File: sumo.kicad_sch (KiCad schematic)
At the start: 51 parts, among them Q1 BPW40, Q2 BPW40, SW1 SW_Push, SW2 SW_DIP_x01, T1 Screw_Terminal_01x04, T2 Screw_Terminal_01x04, T3 Screw_Terminal_01x04, T4 Screw_Terminal_01x04, T5 Screw_Terminal_01x04, U1 PIC16F628A-IP, U2 L7805, U3 L293D, U4 74HC04, U5 TSOP4038, U6 TSOP4038

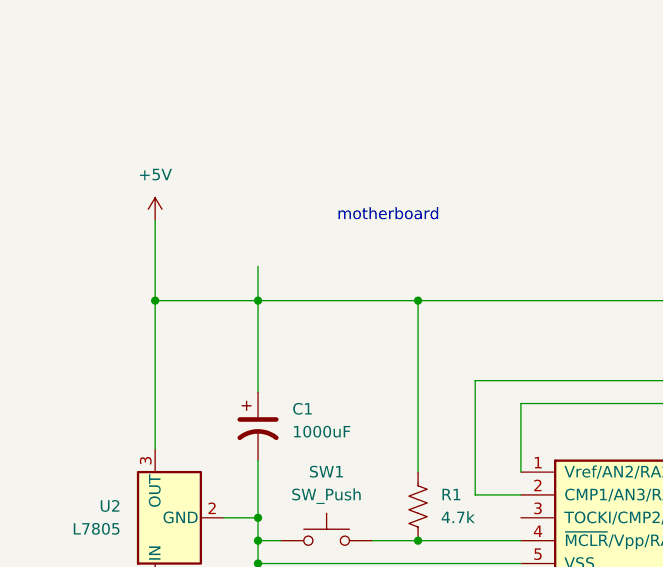
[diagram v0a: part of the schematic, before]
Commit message: motor driver
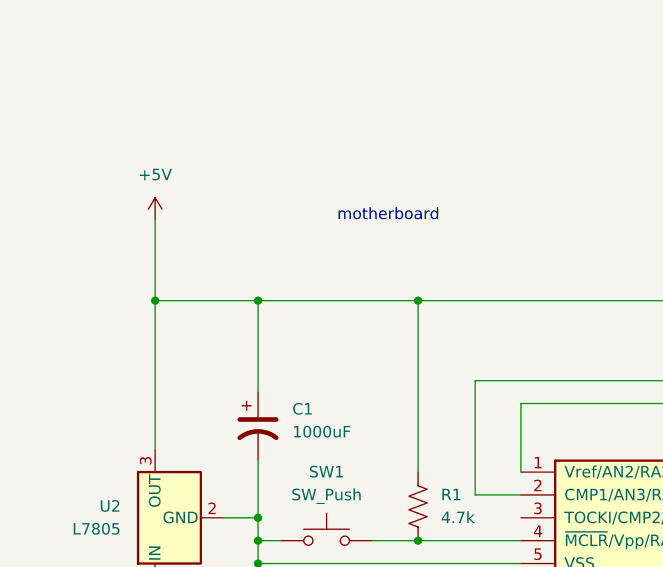
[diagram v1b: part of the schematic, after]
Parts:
- BT1, BT2, BT3: footprint (none) -> Battery:Battery_Pads
- C1: footprint Button_Switch_THT:SW_PUSH_1P1T_6x3.5mm_H5.0_APEM_MJTP1250 -> Capacitor_THT:C_Radial_D10.0mm_H12.5mm_P5.00mm
- SW2: footprint Button_Switch_SMD:SW_DIP_SPSTx01_Slide_9.78x4.72mm_W8.61mm_P2.54mm -> Button_Switch_THT:SW_DIP_SPSTx01_Slide_9.78x4.72mm_W7.62mm_P2.54mm
- T1, T2, T3, T4, T5: footprint TerminalBlock:TerminalBlock_bornier-4_P5.08mm -> TerminalBlock_MetzConnect:TerminalBlock_MetzConnect_Type086_RT03404HBLC_1x04_P3.81mm_Horizontal
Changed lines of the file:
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@@
 	(wire
 		(pts
-			(xy 39.37 138.43) (xy 39.37 134.62)
-		)
-		(stroke
-			(width 0)
-			(type default)
-		)
-	)
-	(wire
-		(pts
 			(xy 186.69 40.64) (xy 196.85 40.64)
 		)
@@
 			)
 		)
-		(property "Footprint" "TerminalBlock:TerminalBlock_bornier-4_P5.08mm"
+		(property "Footprint" "TerminalBlock_MetzConnect:TerminalBlock_MetzConnect_Type086_RT03404HBLC_1x04_P3.81mm_Horizontal"
 			(at 63.5 172.72 0)
 			(effects
@@
 			)
 		)
-		(property "Footprint" ""
+		(property "Footprint" "Battery:Battery_Pads"
 			(at 25.4 68.326 90)
 			(effects
@@
 			)
 		)
-		(property "Footprint" "TerminalBlock:TerminalBlock_bornier-4_P5.08mm"
+		(property "Footprint" "TerminalBlock_MetzConnect:TerminalBlock_MetzConnect_Type086_RT03404HBLC_1x04_P3.81mm_Horizontal"
 			(at 158.75 190.5 0)
 			(effects
@@
 			)
 		)
-		(property "Footprint" "Button_Switch_SMD:SW_DIP_SPSTx01_Slide_9.78x4.72mm_W8.61mm_P2.54mm"
+		(property "Footprint" "Button_Switch_THT:SW_DIP_SPSTx01_Slide_9.78x4.72mm_W7.62mm_P2.54mm"
 			(at 123.19 125.73 0)
 			(effects
@@
 			)
 		)
-		(property "Footprint" ""
+		(property "Footprint" "Battery:Battery_Pads"
 			(at 112.014 125.73 90)
 			(effects
@@
 			)
 		)
-		(property "Footprint" "Button_Switch_THT:SW_PUSH_1P1T_6x3.5mm_H5.0_APEM_MJTP1250"
+		(property "Footprint" "Capacitor_THT:C_Radial_D10.0mm_H12.5mm_P5.00mm"
 			(at 39.37 152.4 0)
 			(effects
@@
 			)
 		)
-		(property "Footprint" ""
+		(property "Footprint" "Battery:Battery_Pads"
 			(at 27.94 178.816 90)
 			(effects
@@
 			)
 		)
-		(property "Footprint" "TerminalBlock:TerminalBlock_bornier-4_P5.08mm"
+		(property "Footprint" "TerminalBlock_MetzConnect:TerminalBlock_MetzConnect_Type086_RT03404HBLC_1x04_P3.81mm_Horizontal"
 			(at 90.17 142.24 0)
 			(effects
@@
 			)
 		)
-		(property "Footprint" "TerminalBlock:TerminalBlock_bornier-4_P5.08mm"
+		(property "Footprint" "TerminalBlock_MetzConnect:TerminalBlock_MetzConnect_Type086_RT03404HBLC_1x04_P3.81mm_Horizontal"
 			(at 92.71 80.01 0)
 			(effects
@@
 			)
 		)
-		(property "Footprint" "TerminalBlock:TerminalBlock_bornier-4_P5.08mm"
+		(property "Footprint" "TerminalBlock_MetzConnect:TerminalBlock_MetzConnect_Type086_RT03404HBLC_1x04_P3.81mm_Horizontal"
 			(at 160.02 111.76 0)
 			(effects
